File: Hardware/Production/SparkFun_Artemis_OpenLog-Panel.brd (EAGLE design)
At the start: 137.2 x 167 mm, 1942 parts, among them J105 CORTEX_JTAG, J106 MICRO-SD, J113 CORTEX_JTAG, J114 MICRO-SD, J121 CORTEX_JTAG, J122 MICRO-SD, J14 CORTEX_JTAG, J16 CORTEX_JTAG, J17 MICRO-SD, J18 MICRO-SD, J25 CORTEX_JTAG, J26 MICRO-SD, J33 CORTEX_JTAG, J34 MICRO-SD, J41 CORTEX_JTAG, J42 MICRO-SD, J49 CORTEX_JTAG, J50 MICRO-SD, J57 CORTEX_JTAG, J58 MICRO-SD, J6 CORTEX_JTAG, J65 CORTEX_JTAG, J66 MICRO-SD, J7 MICRO-SD, J73 CORTEX_JTAG, J74 MICRO-SD, J81 CORTEX_JTAG, J82 MICRO-SD, J89 CORTEX_JTAG, J90 MICRO-SD, J97 CORTEX_JTAG, J98 MICRO-SD, Q1 20V/0.2A/8MHz/1.2Ω/1Vth, Q10 20V/0.2A/8MHz/1.2Ω/1Vth, Q100 20V/0.2A/8MHz/1.2Ω/1Vth, Q101 20V/0.2A/8MHz/1.2Ω/1Vth, Q102 20V/0.2A/8MHz/1.2Ω/1Vth, Q103 20V/0.2A/8MHz/1.2Ω/1Vth, Q104 20V/4.2A/52mΩ/1.4W, Q105 20V/4.2A/52mΩ/1.4W, Q106 20V/0.2A/8MHz/1.2Ω/1Vth, Q107 20V/0.2A/8MHz/1.2Ω/1Vth, Q108 20V/0.2A/8MHz/1.2Ω/1Vth, Q109 20V/0.2A/8MHz/1.2Ω/1Vth, Q11 20V/0.2A/8MHz/1.2Ω/1Vth, Q110 20V/0.2A/8MHz/1.2Ω/1Vth, Q111 20V/4.2A/52mΩ/1.4W, Q112 20V/4.2A/52mΩ/1.4W, Q12 20V/0.2A/8MHz/1.2Ω/1Vth, Q13 20V/4.2A/52mΩ/1.4W, Q14 20V/4.2A/52mΩ/1.4W, Q15 20V/0.2A/8MHz/1.2Ω/1Vth, Q16 20V/0.2A/8MHz/1.2Ω/1Vth, Q17 20V/0.2A/8MHz/1.2Ω/1Vth, Q18 20V/0.2A/8MHz/1.2Ω/1Vth, Q19 20V/0.2A/8MHz/1.2Ω/1Vth, Q2 20V/4.2A/52mΩ/1.4W, Q20 20V/4.2A/52mΩ/1.4W, Q21 20V/4.2A/52mΩ/1.4W, Q22 20V/0.2A/8MHz/1.2Ω/1Vth, Q23 20V/0.2A/8MHz/1.2Ω/1Vth, Q24 20V/0.2A/8MHz/1.2Ω/1Vth, Q25 20V/0.2A/8MHz/1.2Ω/1Vth, Q26 20V/0.2A/8MHz/1.2Ω/1Vth, Q27 20V/4.2A/52mΩ/1.4W, Q28 20V/4.2A/52mΩ/1.4W, Q29 20V/0.2A/8MHz/1.2Ω/1Vth, Q3 20V/0.2A/8MHz/1.2Ω/1Vth, Q30 20V/0.2A/8MHz/1.2Ω/1Vth, Q31 20V/0.2A/8MHz/1.2Ω/1Vth, Q32 20V/0.2A/8MHz/1.2Ω/1Vth, Q33 20V/0.2A/8MHz/1.2Ω/1Vth, Q34 20V/4.2A/52mΩ/1.4W, Q35 20V/4.2A/52mΩ/1.4W, Q36 20V/0.2A/8MHz/1.2Ω/1Vth, Q37 20V/0.2A/8MHz/1.2Ω/1Vth, Q38 20V/0.2A/8MHz/1.2Ω/1Vth, Q39 20V/0.2A/8MHz/1.2Ω/1Vth, Q4 20V/4.2A/52mΩ/1.4W, Q40 20V/0.2A/8MHz/1.2Ω/1Vth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

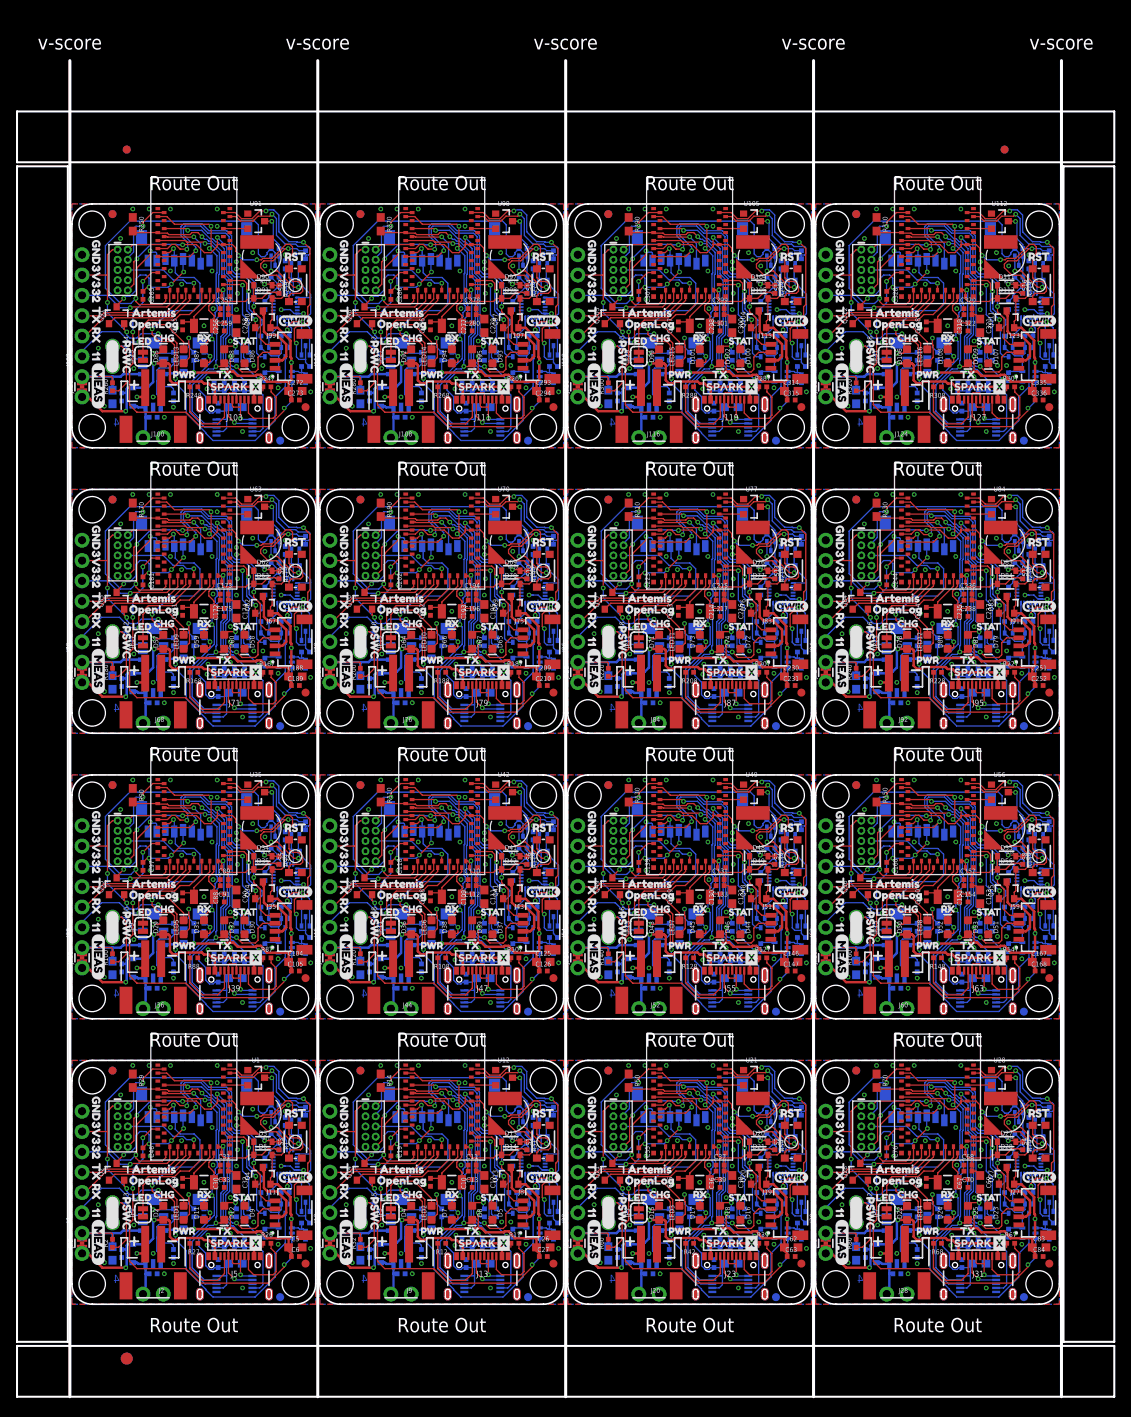
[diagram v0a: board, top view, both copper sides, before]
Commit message: Added production files
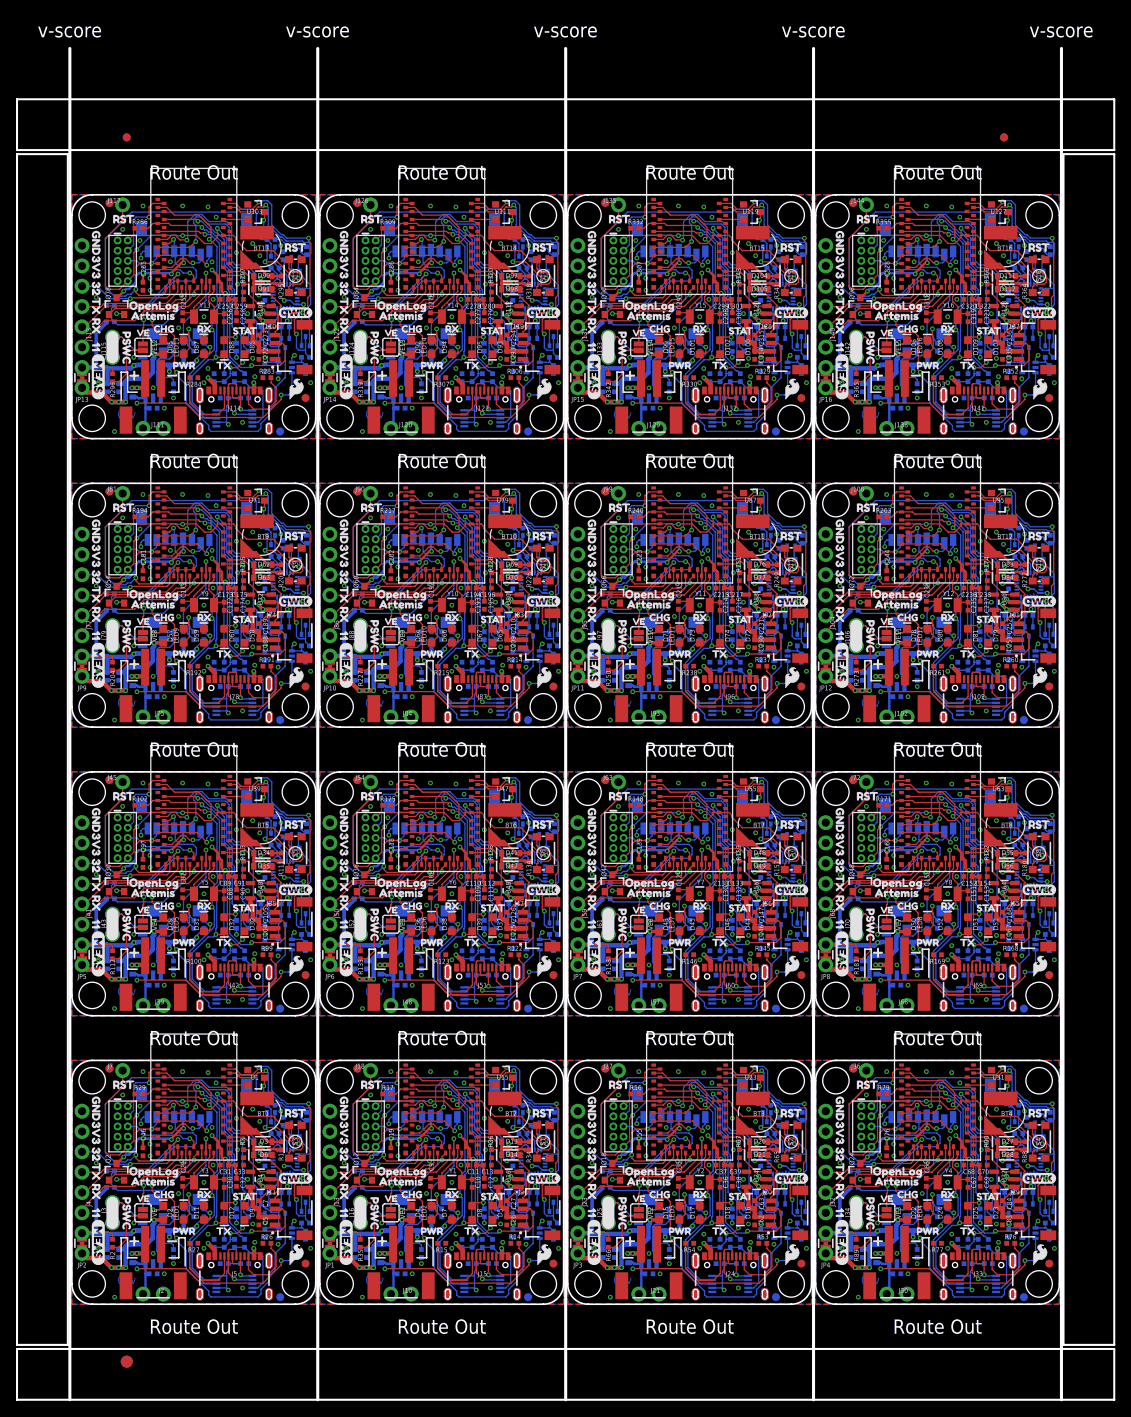
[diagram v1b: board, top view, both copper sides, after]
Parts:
- removed JP17, JP19, JP21, JP23, JP25, JP27, JP29, JP31: (no value), SparkFun-Jumpers:SMT-JUMPER_2_NC_TRACE_SILK
- removed JP18, JP20, JP22, JP24, JP26, JP28, JP30, JP32: MEAS, SparkFun-Jumpers:COMBO-JUMPER_2_NC_TRACE
- removed Q100, Q101, Q102, Q103, Q106, Q107, Q108, Q109, Q110, Q99: 20V/0.2A/8MHz/1.2Ω/1Vth, SparkFun-DiscreteSemi:SOT-416FL
- removed Q104, Q105, Q111, Q112, Q97, Q98: 20V/4.2A/52mΩ/1.4W, SparkFun-DiscreteSemi:SOT23-3
- added J129, J138: (no value), SparkFun-Connectors:JST-2-SMD
- added J130, J133, J139, J142: (no value), SparkFun-Connectors:1X02_NO_SILK
- added J131, J140: (no value), SparkFun-Connectors:1X06_NO_SILK
- added J132, J141: (no value), USBC:USB-C-16P-5
- added J134, J143: MICRO-SD, SparkFun-Connectors:MICRO-SD-SOCKET
- added J135, J144: (no value), SparkFun-Connectors:1X01_NO_SILK
- added J136: CORTEX_JTAG, SparkFun-Connectors:2X5-PTH-1.27MM
- added J137: (no value), SparkFun-Connectors:JST04_1MM_RA
- added LOGO17, LOGO21, LOGO25, LOGO29, LOGO33, LOGO37, LOGO41, LOGO45, LOGO49, LOGO53, LOGO57, LOGO61: OSHW-LOGOS, SparkFun-Aesthetics:OSHW-LOGO-S
- added LOGO18, LOGO20, LOGO22, LOGO24, LOGO26, LOGO28, LOGO30, LOGO32, LOGO34, LOGO36, LOGO38, LOGO40, LOGO42, LOGO44, LOGO46, LOGO48, LOGO50, LOGO52, LOGO54, LOGO56, LOGO58, LOGO60, LOGO62, LOGO64: SFE_LOGO_FLAME.1_INCH, SparkFun-Aesthetics:SFE_LOGO_FLAME_.1
- added LOGO19, LOGO23, LOGO27, LOGO31, LOGO35, LOGO39, LOGO43, LOGO47, LOGO51, LOGO55, LOGO59, LOGO63: SFE_LOGO_NAME.1_INCH, SparkFun-Aesthetics:SFE_LOGO_NAME_.1
- added R321, R344, R367: 1M, New_Parts:0402-TIGHT
- added R322, R345, R368: 2M, New_Parts:0402-TIGHT
- added R323, R333, R334, R335, R336, R337, R338, R339, R346, R356, R357, R358, R359, R360, R361, R362: 2.2k, SparkFun-Resistors:0402-TIGHT
- added R324, R325, R326, R327, R328, R341, R347, R348, R349, R350, R351, R364: 1k, SparkFun-Resistors:0402-TIGHT
- added R329, R330, R352, R353: 5.1k, SparkFun-Resistors:0402-TIGHT
- added R331, R354: 100k, SparkFun-Resistors:0402-TIGHT
- added R332, R355: 220KOHM-0402T-1/16W-1%, SparkFun-Resistors:0402-TIGHT
- added R340, R363: DNP, SparkFun-Resistors:0402-TIGHT
- added R342, R365: 330K, New_Parts:0402-TIGHT
- added R343, R366: 220k, SparkFun-Resistors:0402-TIGHT
- added U$577: (no value), buzzard_labels (14):3V34
- added U$578, U$579: (no value), buzzard_labels (14):113
- added U$580, U$581: (no value), buzzard_labels (14):322
- added U$582, U$583: (no value), buzzard_labels (14):GND5
- added U$584, U$585: (no value), buzzard_labels (14):RX1
- added U$586, U$587: (no value), buzzard_labels (14):TX0
- added U$588, U$589: (no value), buzzard_labels:PSWC0
- added U$590: (no value), buzzard_labels (19):VE0
- added U$591, U$592: (no value), RST_04:RST0
- added U113, U121: MCP73831, SparkFun-IC-Power:SOT23-5
- added U114, U122: ARTEMIS_MODULE, SparkFun-IC-Microcontroller:ARTEMIS_FP
- added U115, U123: CH340E, SparkFun-IC-Comms:MSOP10
- added U116, U124: ICM-20948, SparkFun-Sensors:QFN24-3X3
- added U117, U125: 1.8V/100mA, SparkFun-IC-Power:SC70
- added U118, U120, U126, U128: AP2112K, SparkFun-IC-Power:SOT23-5
- added U119, U127: 3.0V Supervisor, SparkFun-IC-Power:SOT23-3
- added VE, VE1, VE10, VE11, VE12, VE13, VE14, VE15, VE2, VE3, VE4, VE5, VE6, VE7, VE8, VE9: (no value), SparkFun-Jumpers:SMT-JUMPER_2_NO_SILK
- C1, C102, C103, C111, C113, C12, C123, C124, C132, C134, C14, C144, C145, C153, C155, C165, C166, C174, C176, C186, C187, C195, C197, C2, C207, C208, C216, C218, C228, C229, C237, C239, C24, C249, C25, C250, C258, C260, C270, C271, C279, C281, C291, C292, C300, C302, C312, C313, C32, C321, C323, C333, C334, C38, C40, C45, C60, C61, C69, C71, C81, C82, C90, C92: device SparkFun-Capacitors:0603 -> SparkFun-Capacitors:0402-TIGHT
- C104, C125, C146, C167, C188, C209, C230, C251, C26, C272, C293, C314, C335, C5, C62, C83: value 10uF -> 0.1uF; device SparkFun-Capacitors:0603 -> SparkFun-Capacitors:0402-TIGHT
- C105, C126, C147, C168, C189, C210, C231, C252, C27, C273, C294, C315, C336, C63, C84: value 1.0uF -> 2.2uF
- C6: value 1.0uF -> 4.7uF
- C7: value 4.7uF -> 2.2uF
- J10, J120, J21, J48, J93: device SparkFun-Connectors:1X02_NO_SILK -> SparkFun-Connectors:JST-2-SMD
- J100, J28: value (none) -> CORTEX_JTAG; device SparkFun-Connectors:JST-2-SMD -> SparkFun-Connectors:2X5-PTH-1.27MM
- J101, J128, J29, J56: device SparkFun-Connectors:1X02_NO_SILK -> SparkFun-Connectors:JST04_1MM_RA
- J102, J30: device SparkFun-Connectors:1X06_NO_SILK -> SparkFun-Connectors:JST-2-SMD
- J103, J31, J79: device USBC:USB-C-16P-5 -> SparkFun-Connectors:1X02_NO_SILK
- J104, J32, J77: device SparkFun-Connectors:1X02_NO_SILK -> SparkFun-Connectors:1X06_NO_SILK
- J105, J33: value CORTEX_JTAG -> (none); device SparkFun-Connectors:2X5-PTH-1.27MM -> USBC:USB-C-16P-5
- J106, J34, J58: value MICRO-SD -> (none); device SparkFun-Connectors:MICRO-SD-SOCKET -> SparkFun-Connectors:1X02_NO_SILK
- J107, J35: value (none) -> MICRO-SD; device SparkFun-Connectors:JST04_1MM_RA -> SparkFun-Connectors:MICRO-SD-SOCKET
- J108, J36: device SparkFun-Connectors:JST-2-SMD -> SparkFun-Connectors:1X01_NO_SILK
- J109, J37, J64: value (none) -> CORTEX_JTAG; device SparkFun-Connectors:1X02_NO_SILK -> SparkFun-Connectors:2X5-PTH-1.27MM
- J110, J38: device SparkFun-Connectors:1X06_NO_SILK -> SparkFun-Connectors:JST04_1MM_RA
- J111, J39: device USBC:USB-C-16P-5 -> SparkFun-Connectors:JST-2-SMD
- J113, J41: value CORTEX_JTAG -> (none); device SparkFun-Connectors:2X5-PTH-1.27MM -> SparkFun-Connectors:1X06_NO_SILK
- J114, J42: value MICRO-SD -> (none); device SparkFun-Connectors:MICRO-SD-SOCKET -> USBC:USB-C-16P-5
- J115, J43, J67: device SparkFun-Connectors:JST04_1MM_RA -> SparkFun-Connectors:1X02_NO_SILK
- J116, J44: value (none) -> MICRO-SD; device SparkFun-Connectors:JST-2-SMD -> SparkFun-Connectors:MICRO-SD-SOCKET
- J117, J45, J72: device SparkFun-Connectors:1X02_NO_SILK -> SparkFun-Connectors:1X01_NO_SILK
- J118, J46: value (none) -> CORTEX_JTAG; device SparkFun-Connectors:1X06_NO_SILK -> SparkFun-Connectors:2X5-PTH-1.27MM
- J119, J47: device USBC:USB-C-16P-5 -> SparkFun-Connectors:JST04_1MM_RA
- J12, J22, J70, J94: device SparkFun-Connectors:1X06_NO_SILK -> SparkFun-Connectors:1X02_NO_SILK
- J121, J16, J25, J49, J97: value CORTEX_JTAG -> (none); device SparkFun-Connectors:2X5-PTH-1.27MM -> SparkFun-Connectors:1X02_NO_SILK
- J122, J50: value MICRO-SD -> (none); device SparkFun-Connectors:MICRO-SD-SOCKET -> SparkFun-Connectors:1X06_NO_SILK
- J123, J51: device SparkFun-Connectors:JST04_1MM_RA -> USBC:USB-C-16P-5
- J124, J52, J76: device SparkFun-Connectors:JST-2-SMD -> SparkFun-Connectors:1X02_NO_SILK
- J125, J53, J80: value (none) -> MICRO-SD; device SparkFun-Connectors:1X02_NO_SILK -> SparkFun-Connectors:MICRO-SD-SOCKET
- J126, J54: device SparkFun-Connectors:1X06_NO_SILK -> SparkFun-Connectors:1X01_NO_SILK
- J127, J55: value (none) -> CORTEX_JTAG; device USBC:USB-C-16P-5 -> SparkFun-Connectors:2X5-PTH-1.27MM
- J13, J23, J95: device USBC:USB-C-16P-5 -> SparkFun-Connectors:1X06_NO_SILK
- J15, J24, J69, J96: device SparkFun-Connectors:1X02_NO_SILK -> USBC:USB-C-16P-5
- J18, J7, J90: value MICRO-SD -> (none); device SparkFun-Connectors:MICRO-SD-SOCKET -> SparkFun-Connectors:1X01_NO_SILK
- J19, J8, J91: value (none) -> CORTEX_JTAG; device SparkFun-Connectors:JST04_1MM_RA -> SparkFun-Connectors:2X5-PTH-1.27MM
- J20, J9, J92: device SparkFun-Connectors:JST-2-SMD -> SparkFun-Connectors:JST04_1MM_RA
- J27, J99: device SparkFun-Connectors:JST04_1MM_RA -> SparkFun-Connectors:1X01_NO_SILK
- J57: value CORTEX_JTAG -> (none); device SparkFun-Connectors:2X5-PTH-1.27MM -> SparkFun-Connectors:JST-2-SMD
- J59: device SparkFun-Connectors:JST04_1MM_RA -> SparkFun-Connectors:1X06_NO_SILK
- J6, J89: value CORTEX_JTAG -> MICRO-SD; device SparkFun-Connectors:2X5-PTH-1.27MM -> SparkFun-Connectors:MICRO-SD-SOCKET
- J60: device SparkFun-Connectors:JST-2-SMD -> USBC:USB-C-16P-5
- J62: value (none) -> MICRO-SD; device SparkFun-Connectors:1X06_NO_SILK -> SparkFun-Connectors:MICRO-SD-SOCKET
- J63: device USBC:USB-C-16P-5 -> SparkFun-Connectors:1X01_NO_SILK
- J65: value CORTEX_JTAG -> (none); device SparkFun-Connectors:2X5-PTH-1.27MM -> SparkFun-Connectors:JST04_1MM_RA
- J66: value MICRO-SD -> (none); device SparkFun-Connectors:MICRO-SD-SOCKET -> SparkFun-Connectors:JST-2-SMD
- J68: device SparkFun-Connectors:JST-2-SMD -> SparkFun-Connectors:1X06_NO_SILK
- J71: value (none) -> MICRO-SD; device USBC:USB-C-16P-5 -> SparkFun-Connectors:MICRO-SD-SOCKET
- J74: value MICRO-SD -> (none); device SparkFun-Connectors:MICRO-SD-SOCKET -> SparkFun-Connectors:JST04_1MM_RA
- J75: device SparkFun-Connectors:JST04_1MM_RA -> SparkFun-Connectors:JST-2-SMD
- J78: device SparkFun-Connectors:1X06_NO_SILK -> USBC:USB-C-16P-5
- J81: value CORTEX_JTAG -> (none); device SparkFun-Connectors:2X5-PTH-1.27MM -> SparkFun-Connectors:1X01_NO_SILK
- J82: value MICRO-SD -> CORTEX_JTAG; device SparkFun-Connectors:MICRO-SD-SOCKET -> SparkFun-Connectors:2X5-PTH-1.27MM
- JP1, JP11, JP13, JP15, JP3, JP5, JP7, JP9: value (none) -> MEAS; device SparkFun-Jumpers:SMT-JUMPER_2_NC_TRACE_SILK -> SparkFun-Jumpers:COMBO-JUMPER_2_NC_TRACE
- LOGO1, LOGO11, LOGO15, LOGO7: value OSHW-LOGOS -> SFE_LOGO_NAME.1_INCH; device SparkFun-Aesthetics:OSHW-LOGO-S -> SparkFun-Aesthetics:SFE_LOGO_NAME_.1
- LOGO10, LOGO12, LOGO14, LOGO16, LOGO4, LOGO5, LOGO6, LOGO8: value OSHW-LOGOS -> SFE_LOGO_FLAME.1_INCH; device SparkFun-Aesthetics:OSHW-LOGO-S -> SparkFun-Aesthetics:SFE_LOGO_FLAME_.1
- Q12, Q18, Q24, Q30, Q36, Q54, Q60, Q66, Q72, Q78, Q96: value 20V/0.2A/8MHz/1.2Ω/1Vth -> 20V/4.2A/52mΩ/1.4W; device SparkFun-DiscreteSemi:SOT-416FL -> SparkFun-DiscreteSemi:SOT23-3
- Q13, Q14, Q20, Q21, Q27, Q28, Q34, Q35, Q4, Q41, Q49, Q55, Q56, Q62, Q63, Q69, Q70, Q76, Q77, Q83, Q91: value 20V/4.2A/52mΩ/1.4W -> 20V/0.2A/8MHz/1.2Ω/1Vth; device SparkFun-DiscreteSemi:SOT23-3 -> SparkFun-DiscreteSemi:SOT-416FL
- R100, R260: value 10k -> 5.1k
- R101, R16, R193, R216, R55, R78: value 2.2k -> 100k
- R102, R125, R263, R286, R79: value 1k -> 220KOHM-0402T-1/16W-1%
- R103, R104, R105, R106, R126, R139, R162, R185, R199, R219, R222, R223, R224, R242, R243, R244, R245, R246, R264, R265, R266, R31, R59, R62, R63, R8, R82, R83, R84, R85, R86: value 1k -> 2.2k
- R107, R108, R127, R128, R208, R247, R267, R268, R287, R288, R39: value 5.1k -> 2.2k
- R109, R129, R149, R269, R289: value 100k -> 2.2k
- R11, R12, R167, R187, R188, R42, R88: value 5.1k -> 1k
- R110: value 220k -> DNP; device SparkFun-Resistors:0603 -> SparkFun-Resistors:0402-TIGHT
- R111, R117, R118, R121, R134, R141, R157, R211, R212, R213, R232, R233, R234, R235, R236, R255, R256, R257, R258, R272, R278, R281, R295, R301, R318, R51, R52, R71, R72, R73, R74, R75, R94, R95, R96, R97, R98: value 2.2k -> 1k
- R112, R135, R158, R181, R273, R296: value 2.2k -> 330K; device SparkFun-Resistors:0402-TIGHT -> New_Parts:0402-TIGHT
- R113, R136, R251, R274, R297, R3: value 2.2k -> 220k
- R114, R137, R252, R275, R298, R91: value 2.2k -> 1M; device SparkFun-Resistors:0402-TIGHT -> New_Parts:0402-TIGHT
- R115, R138, R161, R253, R276, R92: value 2.2k -> 2M; device SparkFun-Resistors:0402-TIGHT -> New_Parts:0402-TIGHT
- R120, R140, R180, R280: value 10k -> 1k
- R122, R123, R145, R146, R283, R284, R306, R99: value 1k -> 5.1k
- R124, R239, R262, R285: value 1k -> 100k
- R13, R189, R209, R249, R43: value 100k -> 1k
- R130, R150, R270, R290, R310, R70: value 220k -> 2.2k; device SparkFun-Resistors:0603 -> SparkFun-Resistors:0402-TIGHT
- R133, R156, R271, R294, R317, R33, R49: value 2.2k -> DNP
- R14: value 220k -> 5.1k; device SparkFun-Resistors:0603 -> SparkFun-Resistors:0402-TIGHT
- R147, R308: value 5.1k -> 100k
- R148: value 5.1k -> 220KOHM-0402T-1/16W-1%
- R15, R191, R192, R214, R215, R237, R238, R261, R53, R54, R76, R77: value 2.2k -> 5.1k
- R159, R182, R205, R36: value 1k -> 220k
- R160: value 10k -> 1M; device SparkFun-Resistors:0402-TIGHT -> New_Parts:0402-TIGHT
- R169: value 100k -> 5.1k
- R17, R171, R194, R217, R56: value 2.2k -> 220KOHM-0402T-1/16W-1%
- R170: value 220k -> 100k; device SparkFun-Resistors:0603 -> SparkFun-Resistors:0402-TIGHT
- R179, R202, R225, R64: value 1k -> DNP
- R183, R206, R37, R6: value 1k -> 1M; device SparkFun-Resistors:0402-TIGHT -> New_Parts:0402-TIGHT
- R184, R299, R38, R7: value 1k -> 2M; device SparkFun-Resistors:0402-TIGHT -> New_Parts:0402-TIGHT
- R190, R210, R50: value 220k -> 1k; device SparkFun-Resistors:0603 -> SparkFun-Resistors:0402-TIGHT
- R2: value 10k -> 330K; device SparkFun-Resistors:0402-TIGHT -> New_Parts:0402-TIGHT
- R200, R220, R300, R32, R60, R80: value 10k -> 2.2k
- R204, R319, R35, R66: value 1k -> 330K; device SparkFun-Resistors:0402-TIGHT -> New_Parts:0402-TIGHT
- R207: value 5.1k -> 2M; device SparkFun-Resistors:0402-TIGHT -> New_Parts:0402-TIGHT
- R227: value 5.1k -> 330K; device SparkFun-Resistors:0402-TIGHT -> New_Parts:0402-TIGHT
- R228, R67: value 5.1k -> 220k
- R229: value 100k -> 1M; device SparkFun-Resistors:0402-TIGHT -> New_Parts:0402-TIGHT
- R230: value 220k -> 2M; device SparkFun-Resistors:0603 -> New_Parts:0402-TIGHT
- R240: value 10k -> 220KOHM-0402T-1/16W-1%
- R248, R87: value 5.1k -> DNP
- R250: value 220k -> 330K; device SparkFun-Resistors:0603 -> New_Parts:0402-TIGHT
- R29: value 220k -> 220KOHM-0402T-1/16W-1%; device SparkFun-Resistors:0603 -> SparkFun-Resistors:0402-TIGHT
- R309: value 100k -> 220KOHM-0402T-1/16W-1%
- R320: value 10k -> 220k
- R68: value 5.1k -> 1M; device SparkFun-Resistors:0402-TIGHT -> New_Parts:0402-TIGHT
- R69: value 100k -> 2M; device SparkFun-Resistors:0402-TIGHT -> New_Parts:0402-TIGHT
- R89: value 100k -> 330K; device SparkFun-Resistors:0402-TIGHT -> New_Parts:0402-TIGHT
- R90: device SparkFun-Resistors:0603 -> SparkFun-Resistors:0402-TIGHT
- U$100, U$136, U$63, U$99: device buzzard_labels (14):GND5 -> buzzard_labels (14):322
- U$101, U$102, U$138, U$65: device buzzard_labels (14):RX1 -> buzzard_labels (14):GND5
- U$103, U$104, U$140, U$67: device buzzard_labels (14):TX0 -> buzzard_labels (14):RX1
- U$105, U$69: value SPARKX-LOGO3 -> (none); device SparkX:SPARKX-SMALL -> buzzard_labels (14):TX0
- U$106, U$142: device buzzard_labels (15):LED0 -> buzzard_labels (14):TX0
- U$109: device buzzard_labels (2):MEAS3 -> buzzard_labels (19):VE0
- U$110, U$296, U$332, U$74: device buzzard_labels (1):X0 -> RST_04:RST0
- U$111, U$147, U$333, U$369: device buzzard_labels (1):Y1 -> RST_04:RST0
- U$112, U$334: device buzzard_labels (1):Z2 -> buzzard_labels (2):MEAS3
- U$113: device buzzard_labels (1):G5 -> buzzard_labels (1):X0
- U$114: device buzzard_labels (1):A4 -> buzzard_labels (1):Y1
- U$115: device buzzard_labels (1):M3 -> buzzard_labels (1):Z2
- U$116: device buzzard_labels (1):X0 -> buzzard_labels (1):G5
- U$117: device buzzard_labels (1):Y1 -> buzzard_labels (1):A4
- U$118: device buzzard_labels (1):Z2 -> buzzard_labels (1):M3
- U$119, U$335: device qwiic#logo#jpg:QWIIC#LOGO#JPG -> buzzard_labels (1):X0
- U$12, U$73: device buzzard_labels (2):MEAS3 -> RST_04:RST0
- U$120, U$336: device buzzard_labels (12):CHG2 -> buzzard_labels (1):Y1
- U$121, U$337: device buzzard_labels (12):PWR0 -> buzzard_labels (1):Z2
- U$122: device buzzard_labels (12):RX4 -> qwiic#logo#jpg:QWIIC#LOGO#JPG
- U$123: device buzzard_labels (12):STAT5 -> buzzard_labels (12):CHG2
- U$124: device buzzard_labels (12):TX3 -> buzzard_labels (12):PWR0
- U$125: device buzzard_labels (13):ARTEMIS13 -> buzzard_labels (12):RX4
- U$126: device buzzard_labels (13):OPENLOG12 -> buzzard_labels (12):STAT5
- U$127: device buzzard_labels (13):RST9 -> buzzard_labels (12):TX3
- U$128: device buzzard_labels (13):VIN8 -> buzzard_labels (13):ARTEMIS13
- U$129, U$166: device buzzard_labels (14):3V34 -> buzzard_labels (13):OPENLOG12
- U$13, U$260: device buzzard_labels (1):X0 -> buzzard_labels (2):MEAS3
- U$130, U$93: device buzzard_labels (14):3V34 -> buzzard_labels (13):RST9
- U$131, U$168: device buzzard_labels (14):113 -> buzzard_labels (13):VIN8
- U$132, U$59, U$95, U$96: device buzzard_labels (14):113 -> buzzard_labels (14):3V34
- U$133, U$169, U$170, U$206: device buzzard_labels (14):322 -> buzzard_labels (14):3V34
- U$134, U$61, U$97, U$98: device buzzard_labels (14):322 -> buzzard_labels (14):113
- U$135, U$171, U$172, U$208: device buzzard_labels (14):GND5 -> buzzard_labels (14):113
- U$137, U$173, U$174, U$210: device buzzard_labels (14):RX1 -> buzzard_labels (14):322
- U$139, U$175, U$176, U$212: device buzzard_labels (14):TX0 -> buzzard_labels (14):GND5
- U$14, U$20, U$261: device buzzard_labels (1):Y1 -> buzzard_labels (1):X0
- U$141, U$177: value SPARKX-LOGO3 -> (none); device SparkX:SPARKX-SMALL -> buzzard_labels (14):RX1
- U$143, U$179, U$180, U$216: device buzzard_labels:PSWC0 -> buzzard_labels (14):TX0
- U$145, U$181: device buzzard_labels (2):MEAS3 -> buzzard_labels:PSWC0
- U$146, U$368: device buzzard_labels (1):X0 -> buzzard_labels (19):VE0
- U$148, U$184, U$370, U$406: device buzzard_labels (1):Z2 -> RST_04:RST0
- U$149: device buzzard_labels (1):G5 -> buzzard_labels (2):MEAS3
- U$15, U$21, U$262: device buzzard_labels (1):Z2 -> buzzard_labels (1):Y1
- U$150: device buzzard_labels (1):A4 -> buzzard_labels (1):X0
- U$151: device buzzard_labels (1):M3 -> buzzard_labels (1):Y1
- U$152: device buzzard_labels (1):X0 -> buzzard_labels (1):Z2
- U$153: device buzzard_labels (1):Y1 -> buzzard_labels (1):G5
- U$154: device buzzard_labels (1):Z2 -> buzzard_labels (1):A4
- U$155: device qwiic#logo#jpg:QWIIC#LOGO#JPG -> buzzard_labels (1):M3
- U$156, U$372: device buzzard_labels (12):CHG2 -> buzzard_labels (1):X0
- U$157, U$373: device buzzard_labels (12):PWR0 -> buzzard_labels (1):Y1
- U$158, U$374: device buzzard_labels (12):RX4 -> buzzard_labels (1):Z2
- U$159: device buzzard_labels (12):STAT5 -> qwiic#logo#jpg:QWIIC#LOGO#JPG
- U$16: device buzzard_labels (1):G5 -> buzzard_labels (1):Z2
- U$160: device buzzard_labels (12):TX3 -> buzzard_labels (12):CHG2
- U$161: device buzzard_labels (13):ARTEMIS13 -> buzzard_labels (12):PWR0
- U$162: device buzzard_labels (13):OPENLOG12 -> buzzard_labels (12):RX4
- U$163: device buzzard_labels (13):RST9 -> buzzard_labels (12):STAT5
- U$164: device buzzard_labels (13):VIN8 -> buzzard_labels (12):TX3
- U$165, U$202: device buzzard_labels (14):3V34 -> buzzard_labels (13):ARTEMIS13
- U$167, U$204: device buzzard_labels (14):113 -> buzzard_labels (13):RST9
- U$17: device buzzard_labels (1):A4 -> buzzard_labels (1):G5
- U$178, U$214: device buzzard_labels (15):LED0 -> buzzard_labels (14):RX1
- U$18: device buzzard_labels (1):M3 -> buzzard_labels (1):A4
- U$182, U$218, U$404, U$440: device buzzard_labels (1):X0 -> buzzard_labels:PSWC0
- U$183, U$405: device buzzard_labels (1):Y1 -> buzzard_labels (19):VE0
- U$185, U$221: device buzzard_labels (1):G5 -> RST_04:RST0
- U$186: device buzzard_labels (1):A4 -> buzzard_labels (2):MEAS3
- U$187: device buzzard_labels (1):M3 -> buzzard_labels (1):X0
- U$188: device buzzard_labels (1):X0 -> buzzard_labels (1):Y1
- U$189: device buzzard_labels (1):Y1 -> buzzard_labels (1):Z2
- U$19: device buzzard_labels (1):X0 -> buzzard_labels (1):M3
- U$190: device buzzard_labels (1):Z2 -> buzzard_labels (1):G5
- U$191: device qwiic#logo#jpg:QWIIC#LOGO#JPG -> buzzard_labels (1):A4
- U$192: device buzzard_labels (12):CHG2 -> buzzard_labels (1):M3
- U$193, U$409: device buzzard_labels (12):PWR0 -> buzzard_labels (1):X0
- U$194, U$410: device buzzard_labels (12):RX4 -> buzzard_labels (1):Y1
- U$195, U$411: device buzzard_labels (12):STAT5 -> buzzard_labels (1):Z2
- U$196: device buzzard_labels (12):TX3 -> qwiic#logo#jpg:QWIIC#LOGO#JPG
- U$197: device buzzard_labels (13):ARTEMIS13 -> buzzard_labels (12):CHG2
- U$198: device buzzard_labels (13):OPENLOG12 -> buzzard_labels (12):PWR0
- U$199: device buzzard_labels (13):RST9 -> buzzard_labels (12):RX4
- U$200: device buzzard_labels (13):VIN8 -> buzzard_labels (12):STAT5
- U$201, U$238: device buzzard_labels (14):3V34 -> buzzard_labels (12):TX3
- U$203, U$240: device buzzard_labels (14):113 -> buzzard_labels (13):OPENLOG12
- U$205, U$242: device buzzard_labels (14):322 -> buzzard_labels (13):VIN8
- U$207, U$243, U$244, U$280: device buzzard_labels (14):GND5 -> buzzard_labels (14):3V34
- U$209, U$245, U$246, U$282: device buzzard_labels (14):RX1 -> buzzard_labels (14):113
- U$211, U$247, U$248, U$284: device buzzard_labels (14):TX0 -> buzzard_labels (14):322
- U$213, U$249: value SPARKX-LOGO3 -> (none); device SparkX:SPARKX-SMALL -> buzzard_labels (14):GND5
- U$215, U$251, U$252, U$288: device buzzard_labels:PSWC0 -> buzzard_labels (14):RX1
- U$217, U$253: device buzzard_labels (2):MEAS3 -> buzzard_labels (14):TX0
- U$219, U$255, U$441, U$477: device buzzard_labels (1):Y1 -> buzzard_labels:PSWC0
- U$22, U$263: device qwiic#logo#jpg:QWIIC#LOGO#JPG -> buzzard_labels (1):Z2
- U$220, U$442: device buzzard_labels (1):Z2 -> buzzard_labels (19):VE0
- U$222, U$258: device buzzard_labels (1):A4 -> RST_04:RST0
- U$223: device buzzard_labels (1):M3 -> buzzard_labels (2):MEAS3
- U$227: device qwiic#logo#jpg:QWIIC#LOGO#JPG -> buzzard_labels (1):G5
- U$228: device buzzard_labels (12):CHG2 -> buzzard_labels (1):A4
- U$229: device buzzard_labels (12):PWR0 -> buzzard_labels (1):M3
- U$23: device buzzard_labels (12):CHG2 -> qwiic#logo#jpg:QWIIC#LOGO#JPG
- U$230, U$446: device buzzard_labels (12):RX4 -> buzzard_labels (1):X0
- U$231, U$447: device buzzard_labels (12):STAT5 -> buzzard_labels (1):Y1
- U$232, U$448: device buzzard_labels (12):TX3 -> buzzard_labels (1):Z2
- U$233: device buzzard_labels (13):ARTEMIS13 -> qwiic#logo#jpg:QWIIC#LOGO#JPG
- U$234: device buzzard_labels (13):OPENLOG12 -> buzzard_labels (12):CHG2
- U$235: device buzzard_labels (13):RST9 -> buzzard_labels (12):PWR0
- U$236: device buzzard_labels (13):VIN8 -> buzzard_labels (12):RX4
- U$237, U$274: device buzzard_labels (14):3V34 -> buzzard_labels (12):STAT5
- U$239, U$276: device buzzard_labels (14):113 -> buzzard_labels (13):ARTEMIS13
- U$24: device buzzard_labels (12):PWR0 -> buzzard_labels (12):CHG2
- U$241, U$278: device buzzard_labels (14):322 -> buzzard_labels (13):RST9
- U$25: device buzzard_labels (12):RX4 -> buzzard_labels (12):PWR0
- U$250, U$286: device buzzard_labels (15):LED0 -> buzzard_labels (14):GND5
- U$254, U$290, U$476, U$512: device buzzard_labels (1):X0 -> buzzard_labels (14):TX0
- U$256, U$292, U$478, U$514: device buzzard_labels (1):Z2 -> buzzard_labels:PSWC0
- U$257: device buzzard_labels (1):G5 -> buzzard_labels (19):VE0
- U$259, U$295: device buzzard_labels (1):M3 -> RST_04:RST0
- U$26: device buzzard_labels (12):STAT5 -> buzzard_labels (12):RX4
- U$264: device buzzard_labels (12):CHG2 -> buzzard_labels (1):G5
- U$265: device buzzard_labels (12):PWR0 -> buzzard_labels (1):A4
- U$266: device buzzard_labels (12):RX4 -> buzzard_labels (1):M3
- U$267, U$483: device buzzard_labels (12):STAT5 -> buzzard_labels (1):X0
- U$268, U$484: device buzzard_labels (12):TX3 -> buzzard_labels (1):Y1
- U$269, U$485: device buzzard_labels (13):ARTEMIS13 -> buzzard_labels (1):Z2
- U$270: device buzzard_labels (13):OPENLOG12 -> qwiic#logo#jpg:QWIIC#LOGO#JPG
- U$271: device buzzard_labels (13):RST9 -> buzzard_labels (12):CHG2
- U$272: device buzzard_labels (13):VIN8 -> buzzard_labels (12):PWR0
- U$273, U$310: device buzzard_labels (14):3V34 -> buzzard_labels (12):RX4
- U$275, U$312: device buzzard_labels (14):113 -> buzzard_labels (12):TX3
- U$277, U$314: device buzzard_labels (14):322 -> buzzard_labels (13):OPENLOG12
- U$279, U$316: device buzzard_labels (14):GND5 -> buzzard_labels (13):VIN8
- U$281, U$317, U$318, U$354: device buzzard_labels (14):RX1 -> buzzard_labels (14):3V34
- U$283, U$319, U$320, U$356: device buzzard_labels (14):TX0 -> buzzard_labels (14):113
- U$285, U$321: value SPARKX-LOGO3 -> (none); device SparkX:SPARKX-SMALL -> buzzard_labels (14):322
- U$287, U$323, U$324, U$360: device buzzard_labels:PSWC0 -> buzzard_labels (14):GND5
- U$289, U$325: device buzzard_labels (2):MEAS3 -> buzzard_labels (14):RX1
- U$29: device buzzard_labels (12):TX3 -> buzzard_labels (12):STAT5
- U$291, U$327, U$513, U$549: device buzzard_labels (1):Y1 -> buzzard_labels (14):TX0
- U$293, U$329: device buzzard_labels (1):G5 -> buzzard_labels:PSWC0
- U$294: device buzzard_labels (1):A4 -> buzzard_labels (19):VE0
- U$297, U$75: device buzzard_labels (1):Y1 -> buzzard_labels (2):MEAS3
- U$298, U$76, U$82: device buzzard_labels (1):Z2 -> buzzard_labels (1):X0
- U$299, U$83: device qwiic#logo#jpg:QWIIC#LOGO#JPG -> buzzard_labels (1):Y1
- U$30: device buzzard_labels (13):ARTEMIS13 -> buzzard_labels (12):TX3
- U$300, U$84: device buzzard_labels (12):CHG2 -> buzzard_labels (1):Z2
- U$301: device buzzard_labels (12):PWR0 -> buzzard_labels (1):G5
- U$302: device buzzard_labels (12):RX4 -> buzzard_labels (1):A4
- U$303: device buzzard_labels (12):STAT5 -> buzzard_labels (1):M3
- U$304, U$520: device buzzard_labels (12):TX3 -> buzzard_labels (1):X0
- U$305, U$521: device buzzard_labels (13):ARTEMIS13 -> buzzard_labels (1):Y1
- U$306, U$522: device buzzard_labels (13):OPENLOG12 -> buzzard_labels (1):Z2
- U$307: device buzzard_labels (13):RST9 -> qwiic#logo#jpg:QWIIC#LOGO#JPG
- U$308: device buzzard_labels (13):VIN8 -> buzzard_labels (12):CHG2
- U$309, U$346: device buzzard_labels (14):3V34 -> buzzard_labels (12):PWR0
- U$31: device buzzard_labels (13):OPENLOG12 -> buzzard_labels (13):ARTEMIS13
- U$311, U$348: device buzzard_labels (14):113 -> buzzard_labels (12):STAT5
- U$313, U$350: device buzzard_labels (14):322 -> buzzard_labels (13):ARTEMIS13
- U$315, U$352: device buzzard_labels (14):GND5 -> buzzard_labels (13):RST9
- U$322, U$358: device buzzard_labels (15):LED0 -> buzzard_labels (14):322
- U$326, U$362, U$548: device buzzard_labels (1):X0 -> buzzard_labels (14):RX1
- U$328, U$364, U$550: device buzzard_labels (1):Z2 -> buzzard_labels (14):TX0
- U$330, U$366: device buzzard_labels (1):A4 -> buzzard_labels:PSWC0
- U$331: device buzzard_labels (1):M3 -> buzzard_labels (19):VE0
- U$338: device buzzard_labels (12):RX4 -> buzzard_labels (1):G5
- U$339: device buzzard_labels (12):STAT5 -> buzzard_labels (1):A4
- U$340: device buzzard_labels (12):TX3 -> buzzard_labels (1):M3
- U$341, U$557: device buzzard_labels (13):ARTEMIS13 -> buzzard_labels (1):X0
- U$342, U$558: device buzzard_labels (13):OPENLOG12 -> buzzard_labels (1):Y1
- U$343, U$559: device buzzard_labels (13):RST9 -> buzzard_labels (1):Z2
- U$344: device buzzard_labels (13):VIN8 -> qwiic#logo#jpg:QWIIC#LOGO#JPG
- U$345, U$382: device buzzard_labels (14):3V34 -> buzzard_labels (12):CHG2
- U$347, U$384: device buzzard_labels (14):113 -> buzzard_labels (12):RX4
- U$349, U$386: device buzzard_labels (14):322 -> buzzard_labels (12):TX3
- U$351, U$388: device buzzard_labels (14):GND5 -> buzzard_labels (13):OPENLOG12
- U$353, U$390: device buzzard_labels (14):RX1 -> buzzard_labels (13):VIN8
- U$355, U$391, U$392, U$428: device buzzard_labels (14):TX0 -> buzzard_labels (14):3V34
- U$357, U$393: value SPARKX-LOGO3 -> (none); device SparkX:SPARKX-SMALL -> buzzard_labels (14):113
- U$359, U$395, U$396, U$432: device buzzard_labels:PSWC0 -> buzzard_labels (14):322
- U$361, U$397: device buzzard_labels (2):MEAS3 -> buzzard_labels (14):GND5
- U$363, U$399: device buzzard_labels (1):Y1 -> buzzard_labels (14):RX1
- U$365, U$401: device buzzard_labels (1):G5 -> buzzard_labels (14):TX0
- U$367, U$403: device buzzard_labels (1):M3 -> buzzard_labels:PSWC0
- U$371: device qwiic#logo#jpg:QWIIC#LOGO#JPG -> buzzard_labels (2):MEAS3
- U$375: device buzzard_labels (12):STAT5 -> buzzard_labels (1):G5
- U$376: device buzzard_labels (12):TX3 -> buzzard_labels (1):A4
- U$377: device buzzard_labels (13):ARTEMIS13 -> buzzard_labels (1):M3
- U$378: device buzzard_labels (13):OPENLOG12 -> buzzard_labels (1):X0
- U$379: device buzzard_labels (13):RST9 -> buzzard_labels (1):Y1
- U$380: device buzzard_labels (13):VIN8 -> buzzard_labels (1):Z2
- U$381, U$418: device buzzard_labels (14):3V34 -> qwiic#logo#jpg:QWIIC#LOGO#JPG
- U$383, U$420: device buzzard_labels (14):113 -> buzzard_labels (12):PWR0
- U$385, U$422: device buzzard_labels (14):322 -> buzzard_labels (12):STAT5
- U$387, U$424: device buzzard_labels (14):GND5 -> buzzard_labels (13):ARTEMIS13
- U$389, U$426: device buzzard_labels (14):RX1 -> buzzard_labels (13):RST9
- U$394, U$430: device buzzard_labels (15):LED0 -> buzzard_labels (14):113
- U$398, U$434: device buzzard_labels (1):X0 -> buzzard_labels (14):GND5
- U$400, U$436: device buzzard_labels (1):Z2 -> buzzard_labels (14):RX1
- U$402, U$438: device buzzard_labels (1):A4 -> buzzard_labels (14):TX0
- U$407, U$443: device qwiic#logo#jpg:QWIIC#LOGO#JPG -> RST_04:RST0
- U$408: device buzzard_labels (12):CHG2 -> buzzard_labels (2):MEAS3
- U$412: device buzzard_labels (12):TX3 -> buzzard_labels (1):G5
- U$413: device buzzard_labels (13):ARTEMIS13 -> buzzard_labels (1):A4
- U$414: device buzzard_labels (13):OPENLOG12 -> buzzard_labels (1):M3
- U$415: device buzzard_labels (13):RST9 -> buzzard_labels (1):X0
- U$416: device buzzard_labels (13):VIN8 -> buzzard_labels (1):Y1
- U$417, U$454: device buzzard_labels (14):3V34 -> buzzard_labels (1):Z2
- U$419, U$456: device buzzard_labels (14):113 -> buzzard_labels (12):CHG2
- U$421, U$458: device buzzard_labels (14):322 -> buzzard_labels (12):RX4
- U$423, U$460: device buzzard_labels (14):GND5 -> buzzard_labels (12):TX3
- U$425, U$462: device buzzard_labels (14):RX1 -> buzzard_labels (13):OPENLOG12
- U$427, U$464: device buzzard_labels (14):TX0 -> buzzard_labels (13):VIN8
- U$429, U$465: value SPARKX-LOGO3 -> (none); device SparkX:SPARKX-SMALL -> buzzard_labels (14):3V34
- U$431, U$467, U$468, U$504: device buzzard_labels:PSWC0 -> buzzard_labels (14):113
- U$433, U$469: device buzzard_labels (2):MEAS3 -> buzzard_labels (14):322
- U$435, U$471: device buzzard_labels (1):Y1 -> buzzard_labels (14):GND5
- U$437, U$473: device buzzard_labels (1):G5 -> buzzard_labels (14):RX1
- U$439, U$475: device buzzard_labels (1):M3 -> buzzard_labels (14):TX0
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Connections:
- net ARTEMIS_D33 renamed SWO
- removed net ARTEMIS_D1: J6.6, U5.~AD33/SWO
- removed net ARTEMIS_D10: U16.~AD31
- removed net ARTEMIS_D11: U16.AD16
- removed net ARTEMIS_D12: U16.AD34
- removed net ARTEMIS_D13: J25.6, U23.~AD33/SWO
- removed net ARTEMIS_D14: U23.~AD29
- removed net ARTEMIS_D15: U23.~AD35
- removed net ARTEMIS_D16: U8.AD16
- removed net ARTEMIS_D17: U23.~AD31
- removed net ARTEMIS_D18: U23.AD16
- removed net ARTEMIS_D19: U23.AD34
- removed net ARTEMIS_D2: U5.~AD29
- removed net ARTEMIS_D20: J33.6, U30.~AD33/SWO
- removed net ARTEMIS_D21: U30.~AD29
- removed net ARTEMIS_D22: U30.~AD35
- removed net ARTEMIS_D23: U30.~AD31
- removed net ARTEMIS_D24: U30.AD16
- removed net ARTEMIS_D25: U30.AD34
- removed net ARTEMIS_D26: J41.6, U37.~AD33/SWO
- removed net ARTEMIS_D27: U37.~AD29
- removed net ARTEMIS_D28: U37.~AD35
- removed net ARTEMIS_D29: U8.~AD29
- removed net ARTEMIS_D3: U5.~AD35
- removed net ARTEMIS_D30: U37.~AD31
- removed net ARTEMIS_D31: U8.~AD31
- removed net ARTEMIS_D32: U37.AD16
- removed net ARTEMIS_D34: U8.AD34
- removed net ARTEMIS_D35: U8.~AD35
- removed net ARTEMIS_D36: U37.AD34
- removed net ARTEMIS_D37: J49.6, U44.~AD33/SWO
- removed net ARTEMIS_D38: U44.~AD29
- removed net ARTEMIS_D39: U44.~AD35
- removed net ARTEMIS_D4: U5.~AD31
- removed net ARTEMIS_D40: U44.~AD31
- removed net ARTEMIS_D41: U44.AD16
- removed net ARTEMIS_D42: U44.AD34
- removed net ARTEMIS_D43: J57.6, U51.~AD33/SWO
- removed net ARTEMIS_D44: U51.~AD29
- removed net ARTEMIS_D45: U51.~AD35
- removed net ARTEMIS_D46: U51.~AD31
- removed net ARTEMIS_D47: U51.AD16
- removed net ARTEMIS_D48: U51.AD34
- removed net ARTEMIS_D49: J65.6, U58.~AD33/SWO
- removed net ARTEMIS_D5: U5.AD16
- removed net ARTEMIS_D50: U58.~AD29
- removed net ARTEMIS_D51: U58.~AD35
- removed net ARTEMIS_D52: U58.~AD31
- removed net ARTEMIS_D53: U58.AD16
- removed net ARTEMIS_D54: U58.AD34
- removed net ARTEMIS_D55: J73.6, U65.~AD33/SWO
- removed net ARTEMIS_D56: U65.~AD29
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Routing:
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- added copper zone on layer 15, net 3.3V
- added copper zone on layer 15, net 3.3V1
- added copper zone on layer 15, net 3.3V10
- added copper zone on layer 15, net 3.3V11
- added copper zone on layer 15, net 3.3V12
- added copper zone on layer 15, net 3.3V13
- added copper zone on layer 15, net 3.3V14
- added copper zone on layer 15, net 3.3V15
- added copper zone on layer 15, net 3.3V2
- added copper zone on layer 15, net 3.3V3
- added copper zone on layer 15, net 3.3V4
- added copper zone on layer 15, net 3.3V5
- added copper zone on layer 15, net 3.3V6
- added copper zone on layer 15, net 3.3V7
- added copper zone on layer 15, net 3.3V8
- added copper zone on layer 15, net 3.3V9
- added copper zone on layer 15, net 5V
- added copper zone on layer 15, net 5V1
- added copper zone on layer 15, net 5V10
- added copper zone on layer 15, net 5V11
- added copper zone on layer 15, net 5V12
- added copper zone on layer 15, net 5V13
- added copper zone on layer 15, net 5V14
- added copper zone on layer 15, net 5V15
- added copper zone on layer 15, net 5V2
- added copper zone on layer 15, net 5V3
- added copper zone on layer 15, net 5V4
- added copper zone on layer 15, net 5V5
- added copper zone on layer 15, net 5V6
- added copper zone on layer 15, net 5V7
- added copper zone on layer 15, net 5V8
- added copper zone on layer 15, net 5V9
- added copper zone on layer 2, net GND
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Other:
- board size 137.2 x 167 mm -> 137.2 x 168.9 mm
- board text added: "v10"
- board text removed: "x04"
